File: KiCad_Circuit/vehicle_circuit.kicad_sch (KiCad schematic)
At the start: 1 part

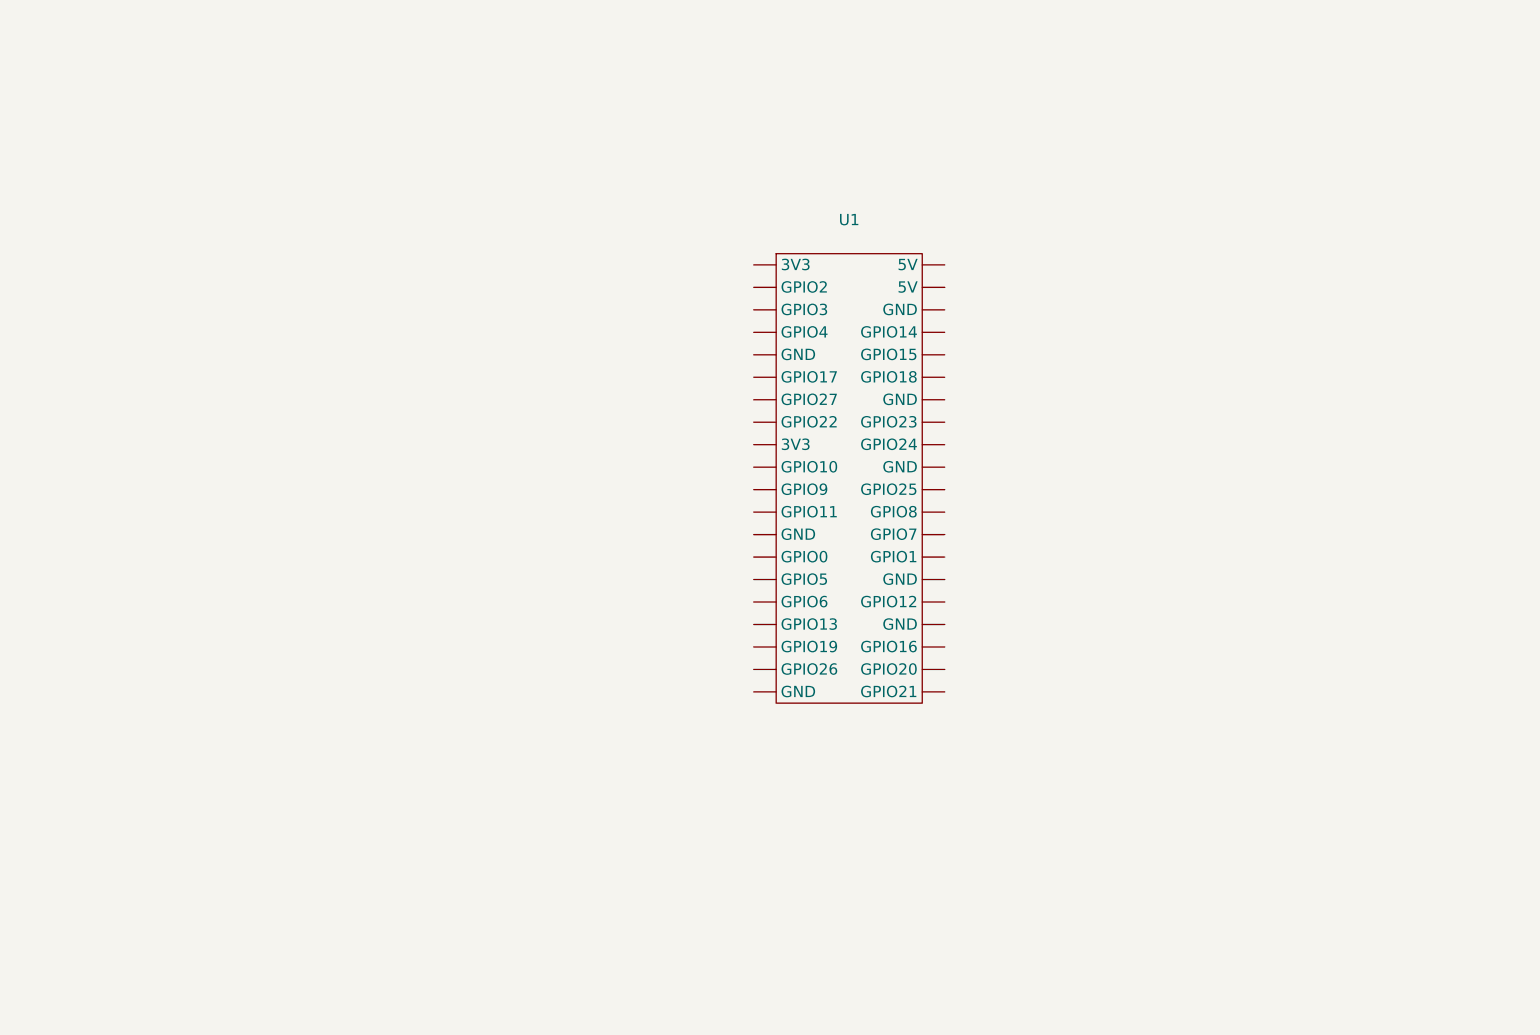
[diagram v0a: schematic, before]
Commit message: Update circuit diagram
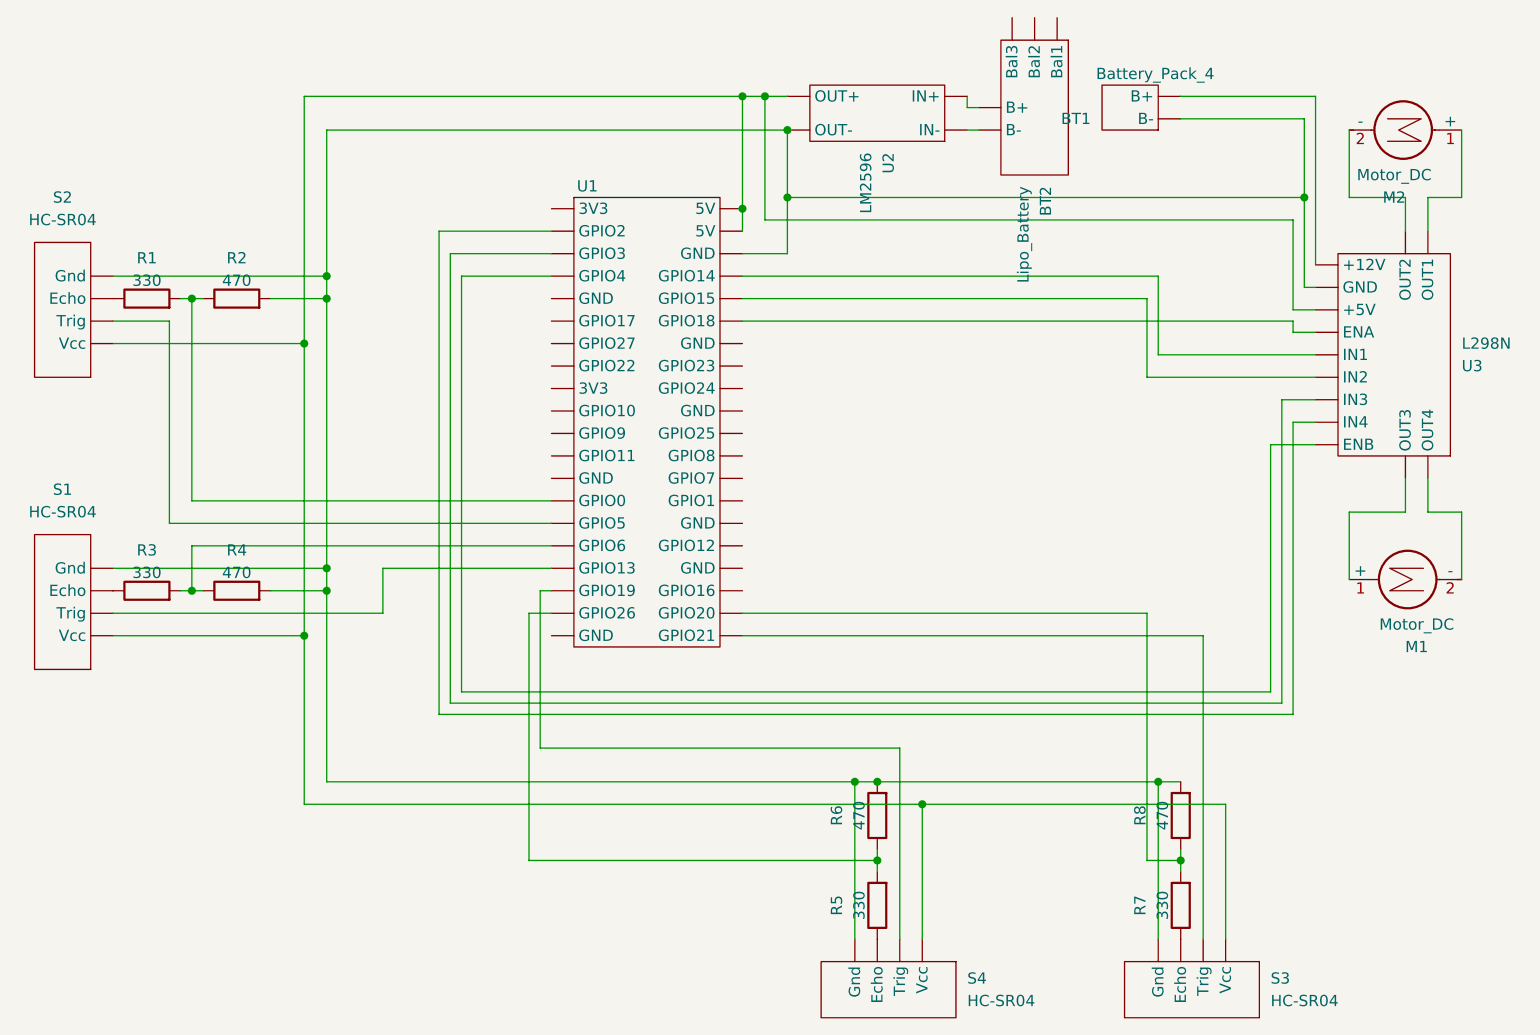
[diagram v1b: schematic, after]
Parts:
- added BT1: Battery_Pack_4, symbol vehicle_circuit:Battery_Pack_4
- added BT2: Lipo_Battery, symbol vehicle_circuit:Lipo_Battery
- added M1, M2: Motor_DC, symbol Motor:Motor_DC
- added R1, R3, R5, R7: 330, symbol Device:R
- added R2, R4, R6, R8: 470, symbol Device:R
- added S1, S2, S3, S4: HC-SR04, symbol vehicle_circuit:HC-SR04
- added U2: LM2596, symbol vehicle_circuit:LM2596
- added U3: L298N, symbol vehicle_circuit:L298N
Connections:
- net at U1. (GPIO9): now also U3. (OUT4)
- new net: R5.2, R6.1, U1. (GPIO9)
- new net: BT1. (B-), R2.2, R4.2, R6.2, R8.2, S1. (Vcc), S2. (Vcc), S3. (Vcc), S4. (Vcc), U1. (GPIO9), U2. (OUT-), U3. (OUT4)
- new net: R3.1, S1. (Vcc)
- new net: R3.2, R4.1, U1. (GPIO9)
- new net: M1.1 (+), U3. (OUT4)
- new net: M1.2 (-), U3. (OUT4)
- new net: S1. (Vcc), S2. (Vcc), S3. (Vcc), S4. (Vcc), U1. (GPIO9), U2. (OUT-), U3. (OUT4)
- new net: S4. (Vcc), U1. (GPIO9)
- new net: R7.2, R8.1, U1. (GPIO9)
- new net: S1. (Vcc), U1. (GPIO9)
- new net: S3. (Vcc), U1. (GPIO9)
- new net: R1.2, R2.1, U1. (GPIO9)
- new net: S2. (Vcc), U1. (GPIO9)
- new net: U1. (GPIO9), U3. (OUT4) (x5)
- new net: M2.1 (+), U3. (OUT4)
- new net: M2.2 (-), U3. (OUT4)
- new net: BT2. (Bal3), U2. (OUT-) (x2)
- new net: BT1. (B-), U3. (OUT4)
- new net: R5.1, S4. (Vcc)
- new net: R7.1, S3. (Vcc)
- new net: R1.1, S2. (Vcc)
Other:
- moved on the sheet: U1
